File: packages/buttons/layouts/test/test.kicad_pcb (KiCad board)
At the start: 2 copper layers, 8 parts

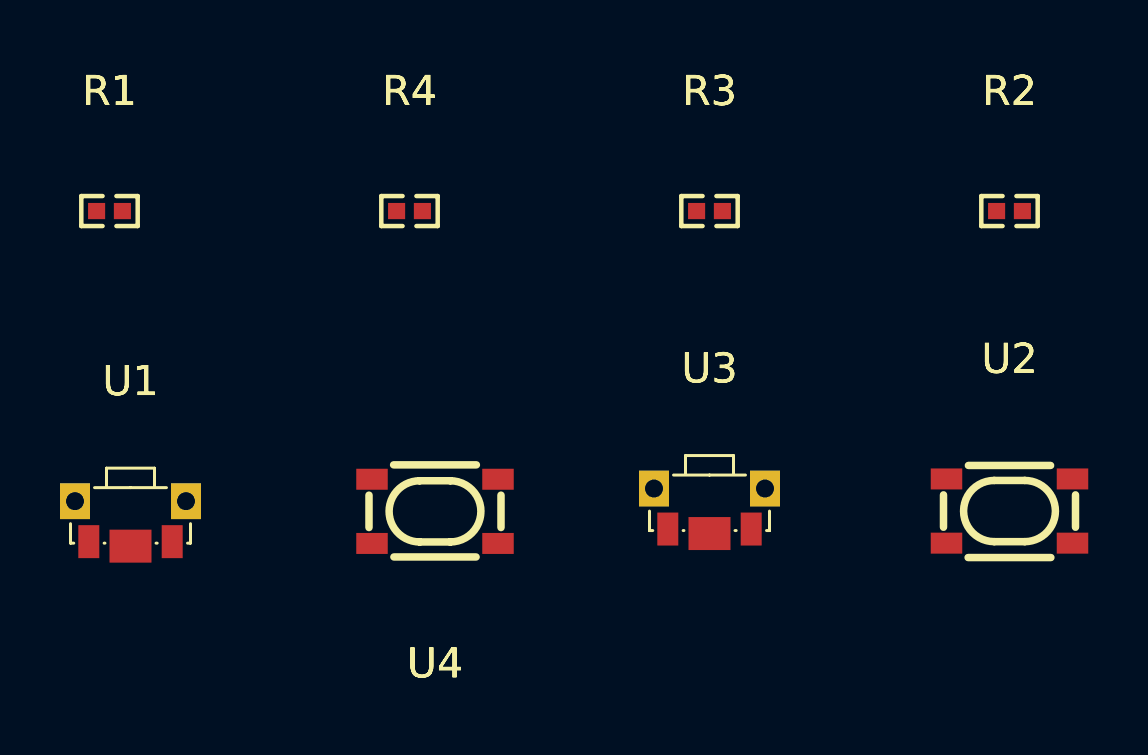
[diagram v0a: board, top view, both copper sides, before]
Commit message: WIP
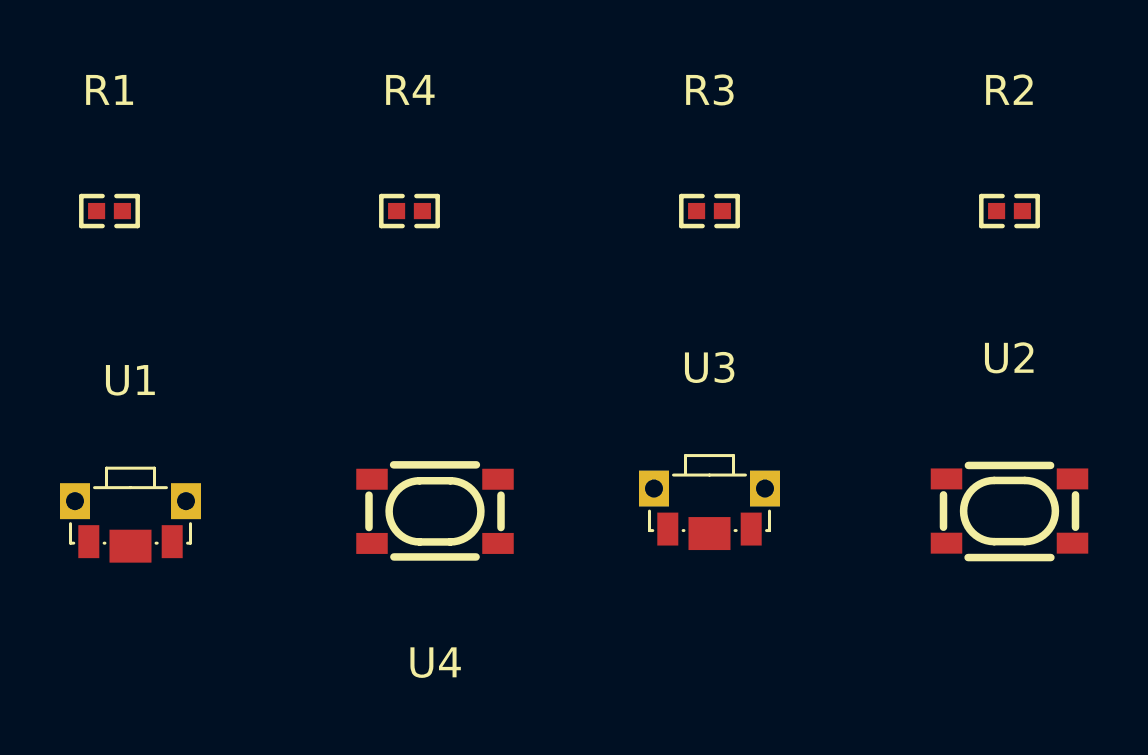
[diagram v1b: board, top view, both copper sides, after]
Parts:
- R1, R2, R3, R4: footprint atopile:R0402-56259e -> UNI_ROYAL_0402WGF1002TCE:R0402
- U1, U3: footprint atopile:KEY-SMD_SKTDLDE010-0426f5 -> ALPSALPINE_SKTDLDE010:KEY-SMD_SKTDLDE010
- U2, U4: footprint atopile:KEY-SMD_4P-L4.2-W3.2-P2.20-LS4.6-a2ccf0 -> ALPSALPINE_SKRPACE010:KEY-SMD_4P-L4.2-W3.2-P2.20-LS4.6
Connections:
- net net renamed _4
- net net-1 renamed _2
- net net-2 renamed unnamed[0]-1
- net net-3 renamed unnamed[0]
- U1 pad 1: line-3 -> line-1
- U2 pad 1: line-1 -> line
- U2 pad 2: line-1 -> line
- U3 pad 1: line -> line-3

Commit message: build all once
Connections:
- net _2 renamed net
- net _4 renamed net-2
- net unnamed[0] renamed net-1
- net unnamed[0]-1 renamed net-3
- U3 pad 1: line-3 -> line-2
- U4 pad 1: line-2 -> line-3
- U4 pad 2: line-2 -> line-3

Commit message: rebuild
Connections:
- net net-3 renamed _3
- R1 pad 1: net-1 -> _2
- R2 pad 1: net-2 -> net
- R3 pad 1: net -> net-1
- U1 pad 1: line-1 -> line-3
- U1 pad 2: net-1 -> _2
- U2 pad 1: line -> line-1
- U2 pad 2: line -> line-1
- U2 pad 3: net-2 -> net
- U2 pad 4: net-2 -> net
- U3 pad 2: net -> net-1
- U4 pad 1: line-3 -> line
- U4 pad 2: line-3 -> line
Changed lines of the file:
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@@
     (net 3 "btn_pulldown_horizontal.btn.footprint.pins[2].net-net")
     (net 4 "btn_pulldown_horizontal-gnd")
-    (net 5 "net-1")
+    (net 5 "_2")
     (net 6 "btn_pulldown_horizontal.btn.footprint.pins[3].net-net")
     (net 7 "btn_pullup_horizontal.btn.footprint.pins[3].net-net")
     (net 8 "line-2")
-    (net 9 "net")
-    (net 10 "line-1")
+    (net 9 "net-1")
+    (net 10 "line-3")
     (net 11 "btn_pullup_horizontal-hv")
     (net 12 "btn_pullup_horizontal.btn.footprint.pins[2].net-net")
-    (net 13 "net-2")
-    (net 14 "line")
-    (net 15 "line-3")
-    (net 16 "net-3")
+    (net 13 "net")
+    (net 14 "line-1")
+    (net 15 "line")
+    (net 16 "_3")
     (footprint "UNI_ROYAL_0402WGF1002TCE:R0402"
         (layer "F.Cu")
@@
             (size 0.57 0.54)
             (layers "F.Cu" "F.Paste" "F.Mask")
-            (net 9 "net")
+            (net 9 "net-1")
         )
         (model "${KIPRJMOD}/../../parts/UNI_ROYAL_0402WGF1002TCE/R0402_L1.0-W0.5-H0.4.step"
@@
             (size 0.7 1.1)
             (layers "F.Cu" "F.Paste" "F.Mask")
-            (net 9 "net")
+            (net 9 "net-1")
         )
         (pad "1" smd rect
@@
             (size 1.05 0.7)
             (layers "F.Cu" "F.Paste" "F.Mask")
-            (net 14 "line")
+            (net 14 "line-1")
         )
         (pad "2" smd rect
@@
             (size 1.05 0.7)
             (layers "F.Cu" "F.Paste" "F.Mask")
-            (net 14 "line")
+            (net 14 "line-1")
         )
         (pad "3" smd rect
@@
             (size 1.05 0.7)
             (layers "F.Cu" "F.Paste" "F.Mask")
-            (net 13 "net-2")
+            (net 13 "net")
         )
         (pad "4" smd rect
@@
             (size 1.05 0.7)
             (layers "F.Cu" "F.Paste" "F.Mask")
-            (net 13 "net-2")
+            (net 13 "net")
         )
         (model "${KIPRJMOD}/../../parts/ALPSALPINE_SKRPACE010/KEY-SMD_4P-L4.2-W3.2-H2.5-LS4.6-P2.2.step"
@@
             (size 0.57 0.54)
             (layers "F.Cu" "F.Paste" "F.Mask")
-            (net 16 "net-3")
+            (net 16 "_3")
         )
         (model "${KIPRJMOD}/../../parts/UNI_ROYAL_0402WGF1002TCE/R0402_L1.0-W0.5-H0.4.step"
@@
             (size 0.7 1.1)
             (layers "F.Cu" "F.Paste" "F.Mask")
-            (net 5 "net-1")
+            (net 5 "_2")
         )
         (pad "1" smd rect
@@
             (size 0.7 1.1)
             (layers "F.Cu" "F.Paste" "F.Mask")
-            (net 10 "line-1")
+            (net 10 "line-3")
         )
         (pad "3" smd rect
@@
             (size 0.57 0.54)
             (layers "F.Cu" "F.Paste" "F.Mask")
-            (net 13 "net-2")
+            (net 13 "net")
         )
         (model "${KIPRJMOD}/../../parts/UNI_ROYAL_0402WGF1002TCE/R0402_L1.0-W0.5-H0.4.step"
@@
             (size 1.05 0.7)
             (layers "F.Cu" "F.Paste" "F.Mask")
-            (net 15 "line-3")
+            (net 15 "line")
         )
         (pad "2" smd rect
@@
             (size 1.05 0.7)
             (layers "F.Cu" "F.Paste" "F.Mask")
-            (net 15 "line-3")
+            (net 15 "line")
         )
         (pad "3" smd rect
@@
             (size 1.05 0.7)
             (layers "F.Cu" "F.Paste" "F.Mask")
-            (net 16 "net-3")
+            (net 16 "_3")
         )
         (pad "4" smd rect
@@
             (size 1.05 0.7)
             (layers "F.Cu" "F.Paste" "F.Mask")
-            (net 16 "net-3")
+            (net 16 "_3")
         )
         (model "${KIPRJMOD}/../../parts/ALPSALPINE_SKRPACE010/KEY-SMD_4P-L4.2-W3.2-H2.5-LS4.6-P2.2.step"
@@
             (size 0.57 0.54)
             (layers "F.Cu" "F.Paste" "F.Mask")
-            (net 5 "net-1")
+            (net 5 "_2")
         )
         (model "${KIPRJMOD}/../../parts/UNI_ROYAL_0402WGF1002TCE/R0402_L1.0-W0.5-H0.4.step"
